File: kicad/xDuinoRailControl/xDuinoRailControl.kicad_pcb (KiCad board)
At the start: 2 copper layers, 46.2 x 25.4 mm, 11 parts, among them J1 Barrel_Jack_Switch, J2 Screw_Terminal_01x02, J3 OLED_SOCKET, U1 DRV8870DDA, U2 MOUDLE-SEEEDUINO-XIAO-ESP32C3, U3 L78L05_SOT89

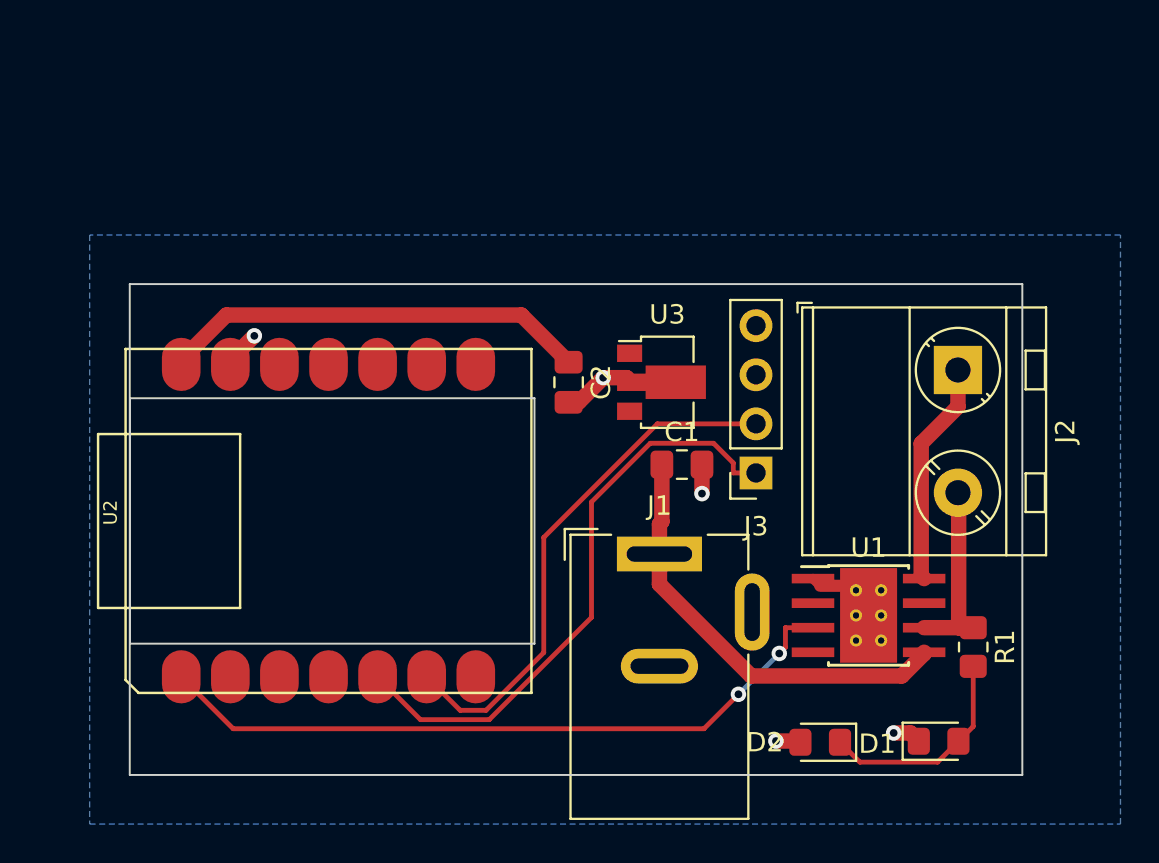
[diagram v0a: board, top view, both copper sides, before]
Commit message: xDuinoRailControl
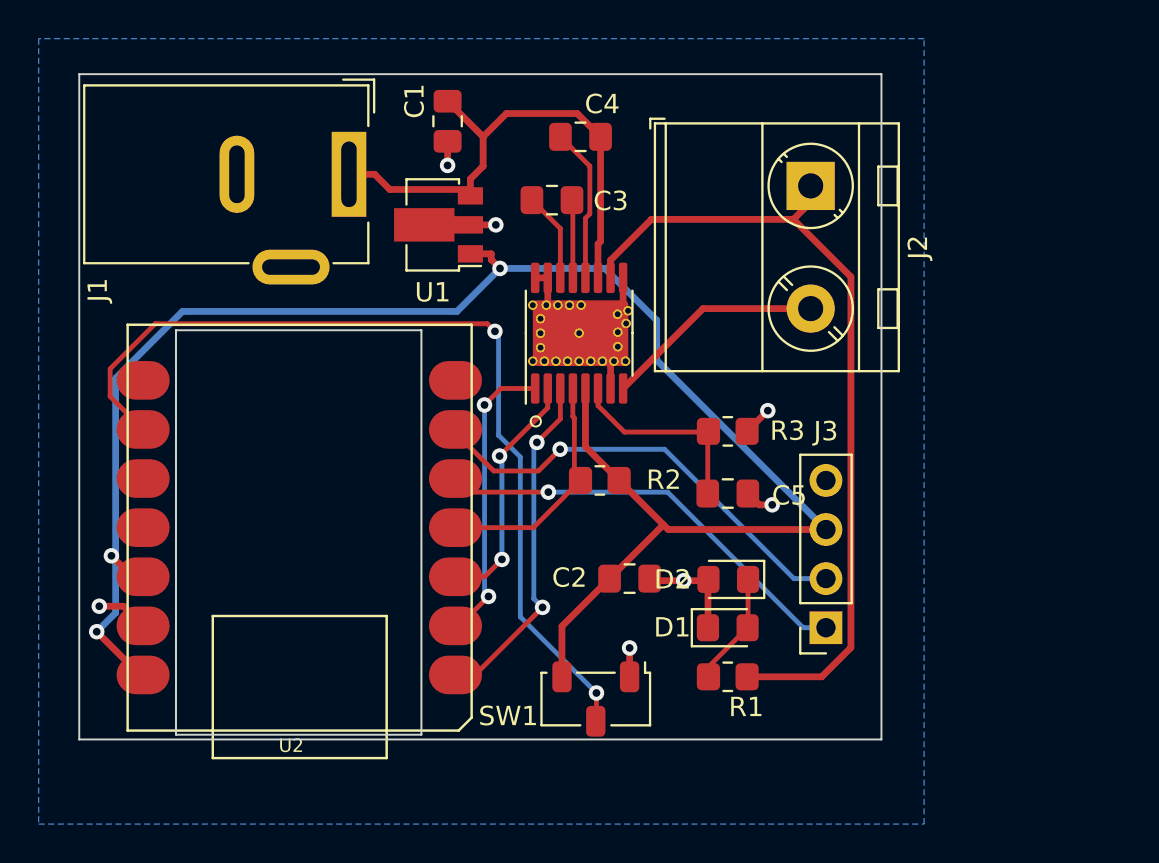
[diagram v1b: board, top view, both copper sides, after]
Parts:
- removed U3: L78L05_SOT89, Package_TO_SOT_SMD:SOT-89-3
- added C3: 22nF, Capacitor_SMD:C_0805_2012Metric_Pad1.18x1.45mm_HandSolder, F.Cu at (135.7, 61.7)
- added C4: 100nF, Capacitor_SMD:C_0805_2012Metric_Pad1.18x1.45mm_HandSolder, F.Cu at (137.2, 58.4)
- added C5: 22nF, Capacitor_SMD:C_0805_2012Metric_Pad1.18x1.45mm_HandSolder, F.Cu at (144.8, 76.9)
- added R2: 47k, Resistor_SMD:R_0805_2012Metric_Pad1.20x1.40mm_HandSolder, F.Cu at (138.2, 76.2)
- added R3: 1k5, Resistor_SMD:R_0805_2012Metric_Pad1.20x1.40mm_HandSolder, F.Cu at (144.8, 73.7)
- added SW1: SW_Nidec_CAS-120A1, Button_Switch_SMD:Nidec_Copal_CAS-120A, F.Cu at (137.9, 87.5)
- added U4: DRV8874PWPR, DRVC8874:HTSSOP-16-1EP_4.4x5mm_P0.65mm_EP3.4x5mm_Mask2.46_HiAmp, F.Cu at (137.1, 68.6)
- R1: value R -> 47k
- U1: value DRV8870DDA -> L78L05_SOT89; footprint Package_SO:Texas_HTSOP-8-1EP_3.9x4.9mm_P1.27mm_EP2.95x4.9mm_Mask2.4x3.1mm_ThermalVias -> Package_TO_SOT_SMD:SOT-89-3
- U2: value MOUDLE-SEEEDUINO-XIAO-ESP32C3 -> XIAO-ESP32C3
- moved U1 30.3 mm to (129.5, 63.0), turned to 180 degrees
- moved J1 25.4 mm to (125.2, 60.4), turned to -90 degrees
- moved C1 21.5 mm to (130.3, 57.6), turned to -90 degrees
- moved U2 19.3 mm to (131.5, 68.1), turned to 180 degrees
- moved R1 12.8 mm to (144.8, 86.4), turned to 180 degrees
- moved D1 12.4 mm to (144.8, 83.8)
- moved J2 12.2 mm to (149.1, 61.0)
- moved C2 10.6 mm to (139.7, 81.3), turned to 0 degrees
- moved D2 9.68 mm to (144.8, 81.3)
- moved J3 8.79 mm to (149.9, 83.8)
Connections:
- C2 pad 1: +5V -> +3V3
- J3 pad 3: +5V -> +3V3
- R1 pad 1: /Power Output/DCC_0 -> /Power Output/DCC_1
- U1 pad 1: GND -> +3V3
- U1 pad 2: unconnected-(U1-IN2-Pad2) -> GND
- U1 pad 3: /Control Board/PWM -> +VIN
- U2 pad 12: unconnected-(U2-3V3-Pad12) -> +3V3
- U2 pad 14: +5V -> +3V3
- U2 pad 9: unconnected-(U2-PA7_A8_D8_SCK-Pad9) -> Net-(SW1-B)
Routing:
- net +3V3: track 0.00 -> 94.4 mm, vias 0 -> 3
- net Net-(SW1-B): track 0.00 -> 47.2 mm, vias 0 -> 2
- net /Power Output/DCC_1: track 11.6 -> 42.7 mm
- net +5V: track 22.2 -> 0.00 mm
- net /Control Board/PWM: track 36.6 -> 18.0 mm
- net /Control Board/BRAKE: track 0.00 -> 15.3 mm, vias 0 -> 2
- net /Control Board/DIRECTION: track 0.00 -> 12.7 mm, vias 0 -> 2
- net /Control Board/SENSE: track 0.00 -> 12.4 mm
- net Net-(U4-IPROPI): track 0.00 -> 10.4 mm
- net /Control Board/SDA: track 30.9 -> 22.4 mm, vias 0 -> 1
- net Net-(U4-VCP): track 0.00 -> 8.02 mm
- net GND: track 13.4 -> 20.9 mm, vias 5 -> 7
- net Net-(D1-A): track 11.2 -> 5.89 mm
- net Net-(U4-CPL): track 0.00 -> 4.63 mm
- net +VIN: track 22.5 -> 27.0 mm
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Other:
- board size 46.2 x 25.4 mm -> 41.5 x 34.4 mm

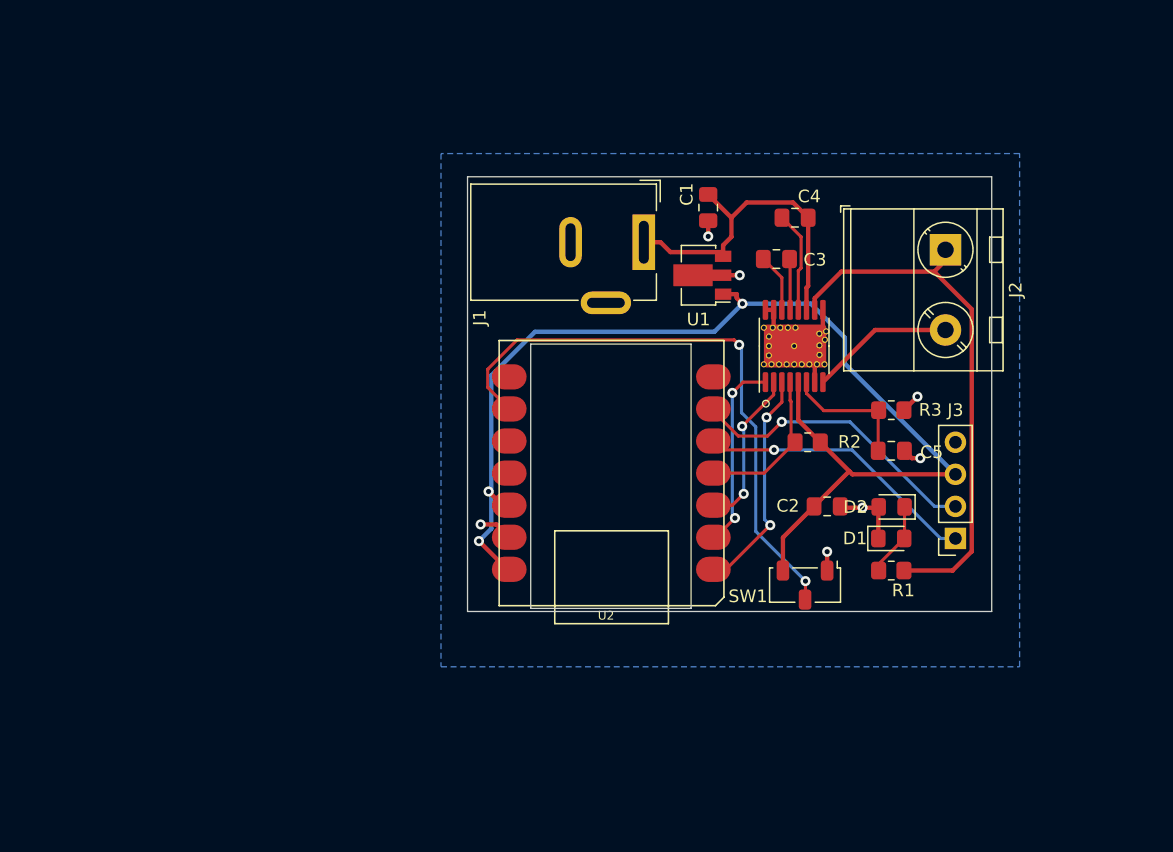
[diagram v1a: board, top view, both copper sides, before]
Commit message: Add encoder
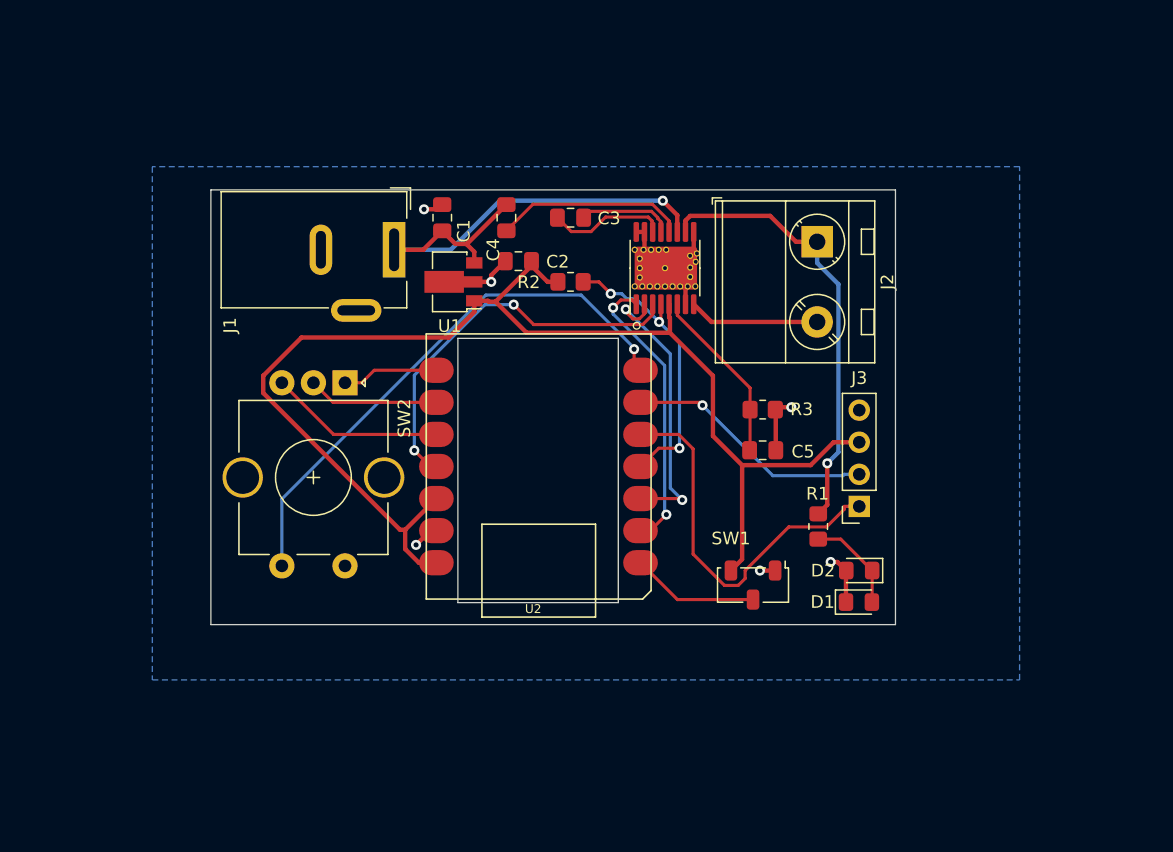
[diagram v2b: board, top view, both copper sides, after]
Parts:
- added SW2: RotaryEncoder_Switch, Rotary_Encoder:RotaryEncoder_Alps_EC11E-Switch_Vertical_H20mm_CircularMountingHoles, F.Cu at (101.5, 71.5)
- moved C2 31.2 mm to (115.3, 61.9), turned to 180 degrees
- moved C4 22.9 mm to (114.3, 58.4), turned to 90 degrees
- moved R2 22.7 mm to (119.4, 63.5), turned to 0 degrees
- moved C1 21.1 mm to (109.2, 58.4), turned to 90 degrees
- moved J1 19.8 mm to (105.4, 61.0)
- moved U1 19.7 mm to (109.8, 63.5)
- moved C3 16.6 mm to (119.4, 58.4)
- moved U4 11.9 mm to (126.9, 62.4)
- moved C5 10.2 mm to (134.6, 76.8)
- moved R3 10.2 mm to (134.6, 73.6)
- moved J2 10.2 mm to (138.9, 60.3)
- moved J3 8.03 mm to (142.2, 81.3)
- moved R1 6.76 mm to (139.0, 82.9), turned to -90 degrees
- moved U2 5.79 mm to (125.8, 67.6)
- moved D1 5.65 mm to (142.2, 88.9)
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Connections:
- U2 pad 1: /Control Board/PWM -> Net-(SW1-B)
- U2 pad 10: unconnected-(U2-PA5_A9_D9_MISO-Pad10) -> Net-(U2-PA5_A9_D9_MISO)
- U2 pad 11: unconnected-(U2-PA6_A10_D10_MOSI-Pad11) -> /Control Board/PWM
- U2 pad 7: unconnected-(U2-PB08_A6_D6_TX-Pad7) -> Net-(U2-PB08_A6_D6_TX)
- U2 pad 8: unconnected-(U2-PB09_A7_D7_RX-Pad8) -> Net-(U2-PB09_A7_D7_RX)
- U2 pad 9: Net-(SW1-B) -> Net-(U2-PA7_A8_D8_SCK)
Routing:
- net Net-(U2-PB08_A6_D6_TX): track 0.00 -> 43.6 mm, vias 0 -> 1
- net Net-(SW1-B): track 47.2 -> 10.1 mm, vias 2 -> 0
- net Net-(U2-PA5_A9_D9_MISO): track 0.00 -> 13.9 mm
- net /Control Board/PWM: track 18.0 -> 31.2 mm
- net +VIN: track 27.0 -> 38.8 mm, vias 0 -> 1
- net /Control Board/SENSE: track 12.4 -> 23.1 mm, vias 0 -> 3
- net /Control Board/DIRECTION: track 12.7 -> 23.1 mm
- net Net-(U2-PA7_A8_D8_SCK): track 0.00 -> 10.4 mm
- net /Control Board/SDA: track 22.4 -> 30.2 mm, vias 1 -> 0
- net +3V3: track 94.4 -> 102.1 mm, vias 3 -> 0
- net Net-(U2-PB09_A7_D7_RX): track 0.00 -> 7.65 mm
- net /Control Board/BRAKE: track 15.3 -> 22.9 mm
- net /Power Output/DCC_1: track 42.7 -> 35.2 mm, vias 0 -> 1
- net Net-(U4-VCP): track 8.02 -> 15.2 mm
- net Net-(U4-CPL): track 4.63 -> 9.45 mm
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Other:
- board size 41.5 x 34.4 mm -> 54.2 x 34.4 mm

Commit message: More improvements
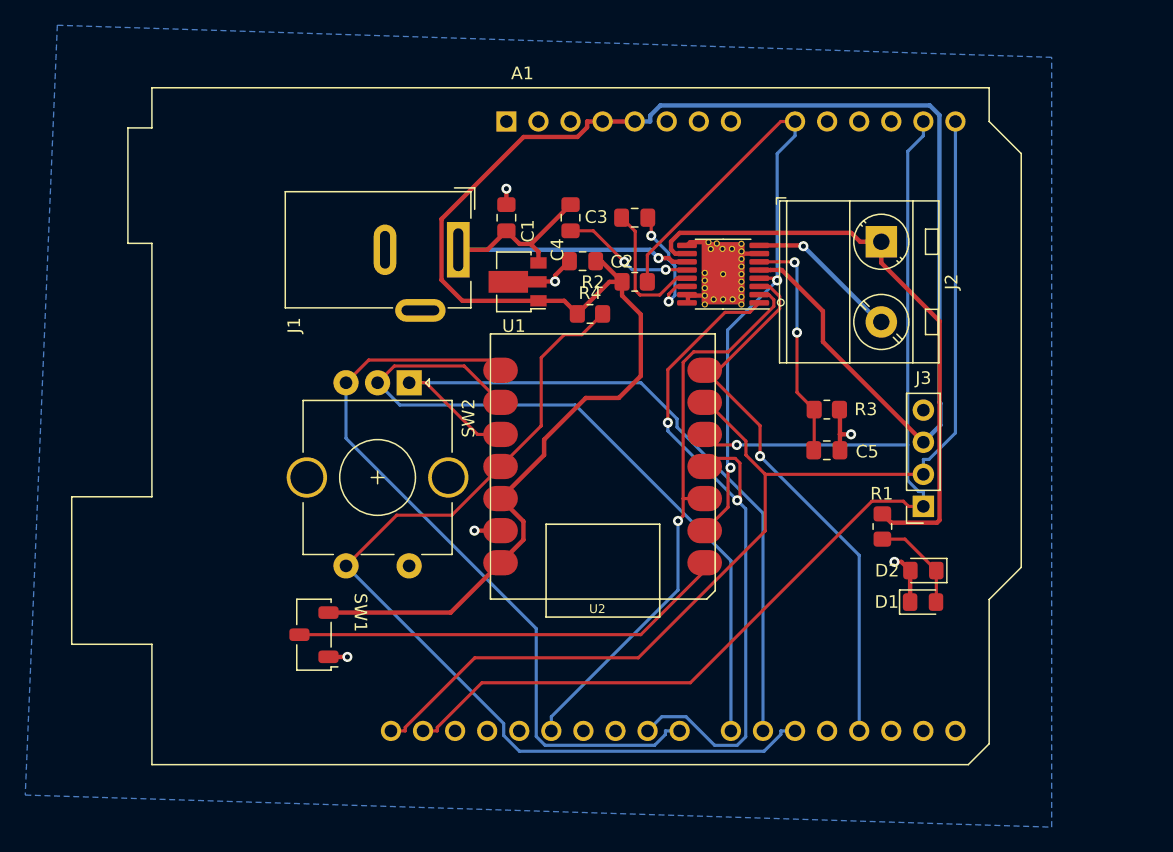
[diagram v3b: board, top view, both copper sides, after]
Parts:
- added A1: Arduino_UNO_R3, Module:Arduino_UNO_R3, F.Cu at (114.3, 50.8)
- added R4: 10k, Resistor_SMD:R_0805_2012Metric_Pad1.20x1.40mm_HandSolder, F.Cu at (120.9, 66.0)
- moved SW1 35.0 mm to (99.1, 91.4), turned to 180 degrees
- moved C2 5.08 mm to (120.3, 61.9)
- moved D1 5.08 mm to (147.3, 88.9)
- moved J2 5.08 mm to (144.0, 60.3)
- moved R1 5.08 mm to (144.1, 82.9)
- moved U2 5.08 mm to (130.8, 67.6)
- moved C1 5.08 mm to (114.3, 58.4)
- moved C3 5.08 mm to (124.5, 58.4), turned to 0 degrees
- moved C4 5.08 mm to (119.4, 58.4)
- moved J1 5.08 mm to (110.5, 61.0)
- moved R2 5.08 mm to (124.5, 63.5)
- moved SW2 5.08 mm to (106.6, 71.5)
- moved U1 5.08 mm to (114.9, 63.5)
- moved C5 5.08 mm to (139.7, 76.8)
- moved D2 5.08 mm to (147.3, 86.4)
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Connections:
- net Net-(U2-PA7_A8_D8_SCK) renamed /Control Board/DC2
- SW2 pad A: Net-(U2-PB09_A7_D7_RX) -> /Control Board/DC1
- SW2 pad B: Net-(U2-PA5_A9_D9_MISO) -> /Control Board/DC3
- SW2 pad S1: Net-(U2-PB08_A6_D6_TX) -> /Control Board/DPU
- U2 pad 10: Net-(U2-PA5_A9_D9_MISO) -> /Control Board/DC1
- U2 pad 11: /Control Board/PWM -> /Control Board/DPU
- U2 pad 2: /Control Board/BRAKE -> /Control Board/SENSE
- U2 pad 4: /Control Board/SENSE -> /Control Board/BRAKE
- U2 pad 7: Net-(U2-PB08_A6_D6_TX) -> /Control Board/PWM
- U2 pad 8: Net-(U2-PB09_A7_D7_RX) -> /Control Board/DC3
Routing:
- net /Control Board/DPU: track 0.00 -> 74.8 mm
- net /Control Board/SCL: track 19.8 -> 90.4 mm, vias 1 -> 0
- net /Control Board/SDA: track 30.2 -> 95.6 mm, vias 0 -> 1
- net /Control Board/DC3: track 0.00 -> 59.9 mm
- net /Control Board/DC1: track 0.00 -> 58.9 mm
- net +3V3: track 102.1 -> 160.4 mm
- net /Control Board/DC2: track 10.4 -> 58.8 mm
- net Net-(U2-PB08_A6_D6_TX): track 43.6 -> 0.00 mm, vias 1 -> 0
- net /Control Board/BRAKE: track 22.9 -> 56.8 mm
- net /Control Board/SENSE: track 23.1 -> 55.3 mm, vias 3 -> 2
- net Net-(SW1-B): track 10.1 -> 34.8 mm
- net /Control Board/DIRECTION: track 23.1 -> 46.1 mm, vias 2 -> 1
- net Net-(U2-PA5_A9_D9_MISO): track 13.9 -> 0.00 mm
- net /Control Board/PWM: track 31.2 -> 44.2 mm, vias 2 -> 1
- net /Power Output/DCC_1: track 35.2 -> 48.1 mm, vias 1 -> 0
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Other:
- board outline removed
